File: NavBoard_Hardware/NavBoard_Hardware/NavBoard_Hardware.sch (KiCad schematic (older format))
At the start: 17 parts, among them U1 OKI-5V, U4 OKI-3V3, U6 Raspberry_Pi

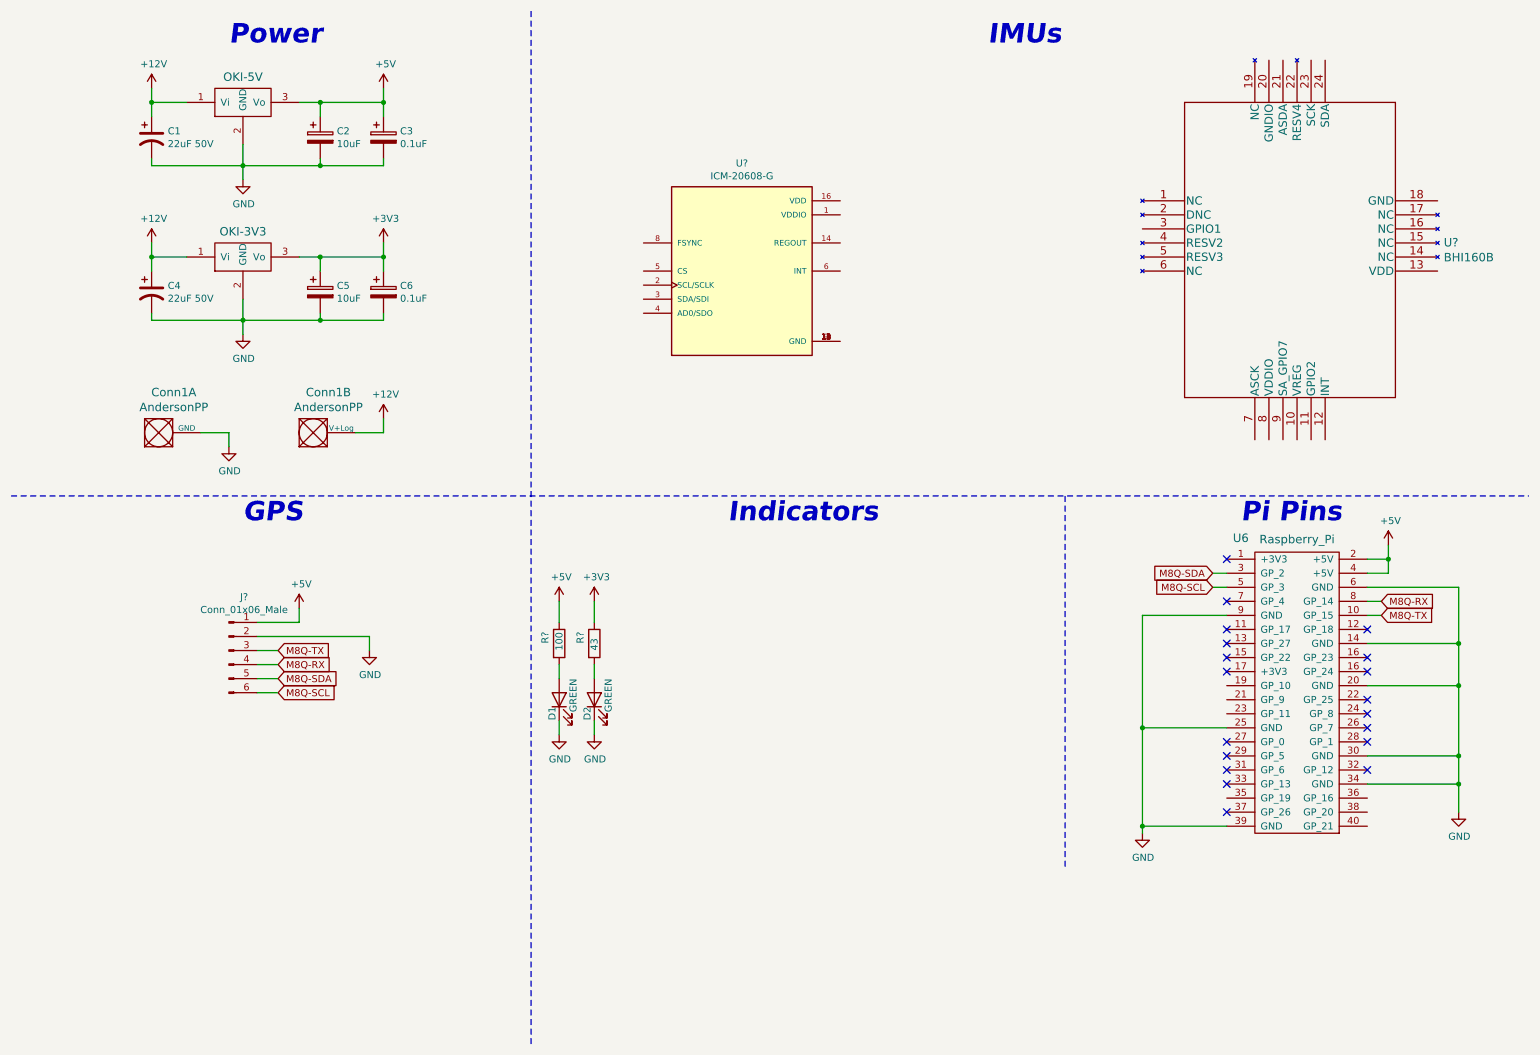
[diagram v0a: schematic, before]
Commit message: Completed schematic
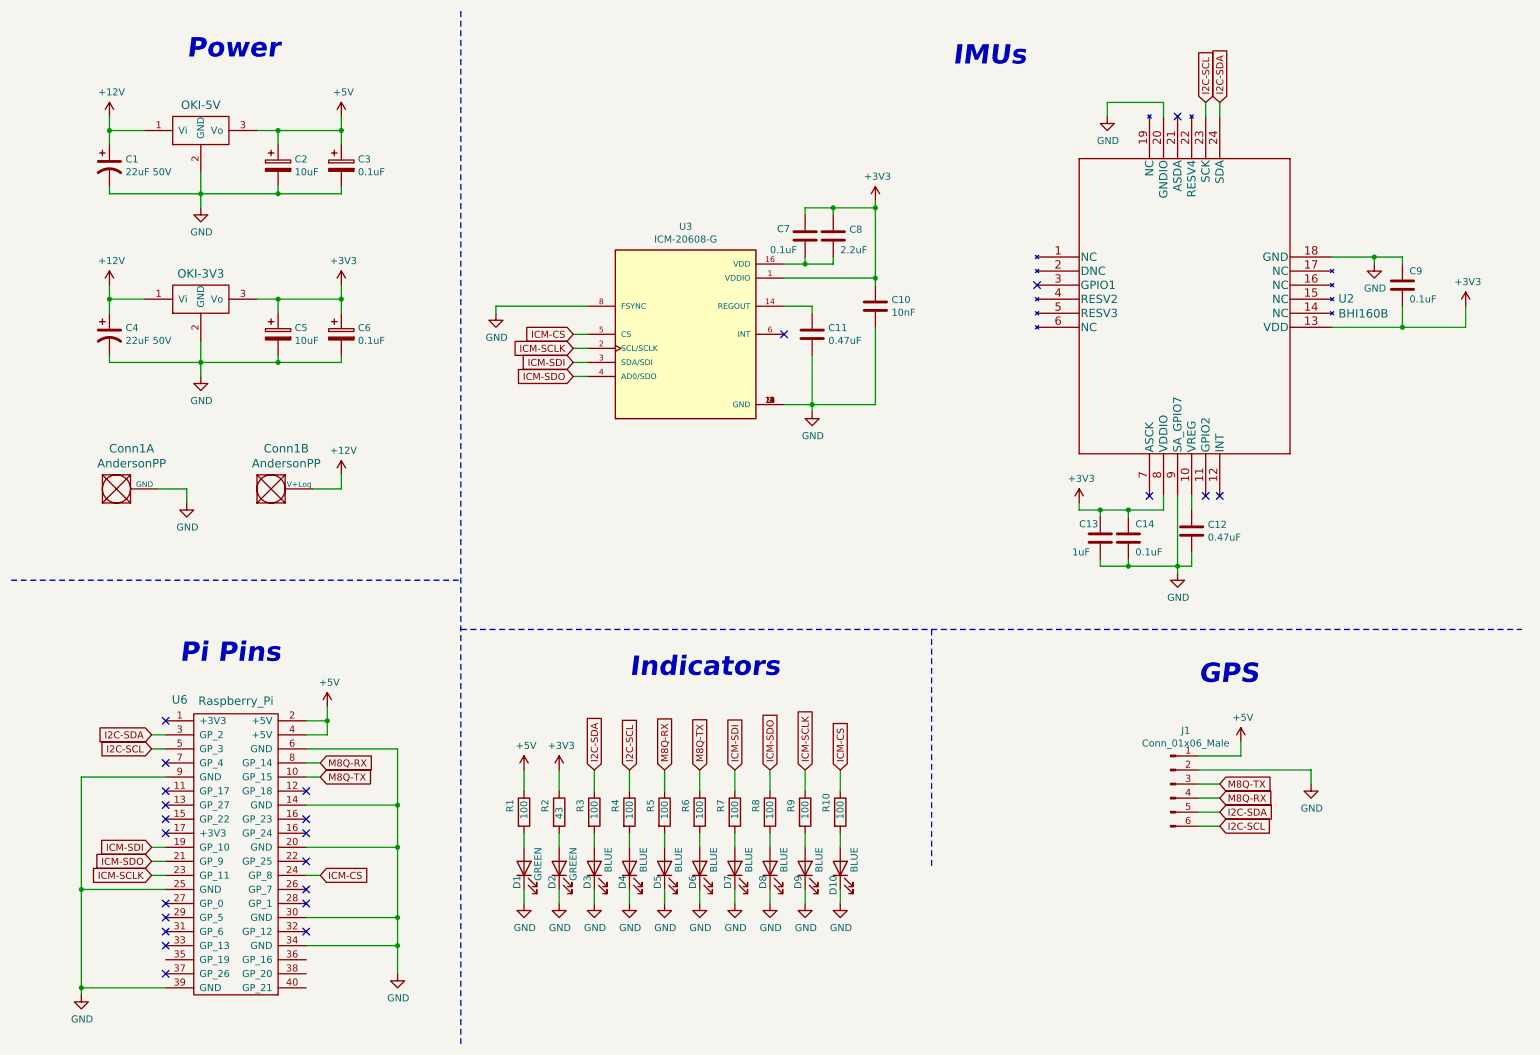
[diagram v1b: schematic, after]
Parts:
- added C10: 10nF, symbol Device:C
- added C11, C12: 0.47uF, symbol Device:C
- added C13: 1uF, symbol Device:C
- added C14, C7, C9: 0.1uF, symbol Device:C
- added C8: 2.2uF, symbol Device:C
- added D10, D3, D4, D5, D6, D7, D8, D9: BLUE, LED_SMD:LED_0603_1608Metric_Pad1.05x0.95mm_HandSolder, symbol Device:LED
- added R10, R3, R4, R5, R6, R7, R8, R9: 100, Resistor_SMD:R_0603_1608Metric_Pad0.98x0.95mm_HandSolder, symbol Device:R
- gave numbers to parts that had none: 5
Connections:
- net M8Q-SCL is gone; now on net I2C-SCL: J1.6 (Pin_6), U6.5 (GP_3)
- net M8Q-SDA is gone; now on net I2C-SDA: J1.5 (Pin_5), U6.3 (GP_2)
- net +3V3: now also U2.13 (VDD), U2.8 (VDDIO), U3.1 (VDDIO), C10.1, C13.1, C14.1, C7.1, C8.1, C9.2
- net GND: now also U2.18 (GND), U2.20 (GNDIO), U2.9 (SA_GPIO7), U3.10 (GND), U3.11 (GND), U3.12 (GND), U3.13 (GND), U3.15 (GND), U3.8 (FSYNC), U3.9 (GND), C10.2, C11.2, C12.2, C13.2, C14.2, C9.1, D10.1 (K), D3.1 (K), D4.1 (K), D5.1 (K), D6.1 (K), D7.1 (K), D8.1 (K), D9.1 (K)
- net M8Q-RX: now also R5.1
- net M8Q-TX: now also R6.1
- net ICM-SDI: now reaches U6.19 (GP_10)
- net ICM-SDI: now also U3.3 (SDA/SDI), R7.1
- net ICM-SDO: now reaches U6.21 (GP_9)
- net ICM-SDO: now also U3.4 (AD0/SDO), R8.1
- net ICM-SCLK: now reaches U6.23 (GP_11)
- net ICM-SCLK: now also U3.2 (SCL/SCLK), R9.1
- net ICM-CS: now reaches U6.24 (GP_8)
- net ICM-CS: now also U3.5 (CS), R10.1
- net at U3.14 (REGOUT): now also C11.1
- net at U3.16 (VDD): now also C7.2, C8.2
- net at U2.10 (VREG): now also C12.1
- net I2C-SCL: now reaches U2.23 (SCK)
- net I2C-SCL: now also R4.1
- net I2C-SDA: now reaches U2.24 (SDA)
- net I2C-SDA: now also R3.1
- new net: D3.2 (A), R3.2
- new net: D4.2 (A), R4.2
- new net: D5.2 (A), R5.2
- new net: D6.2 (A), R6.2
- new net: D7.2 (A), R7.2
- new net: D8.2 (A), R8.2
- new net: D9.2 (A), R9.2
- new net: D10.2 (A), R10.2
- no-connect marks 19 -> 24
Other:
- moved on the sheet: C1, C2, C3, C4, C5, C6, Conn1A, Conn1B, D1, D2, J1, R1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
